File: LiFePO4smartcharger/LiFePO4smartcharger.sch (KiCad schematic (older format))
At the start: 105 parts, among them J1 Conn_01x02, J10 Conn_01x01, J11 Conn_01x01, J12 Conn_01x04, J13 Conn_01x01, J2 Conn_02x03_Odd_Even, J3 Conn_01x02, J4 Conn_01x02, J5 Barrel_Jack, J6 Conn_01x01, J7 Conn_01x01, J8 Conn_01x02, J9 Conn_01x02, Q1 TIP42, Q2 TIP41, Q3 2N3906, Q4 TIP41C, T1 Transformer_1P1Sdotted, U1 ATMEGA328P-PU, U2 LM358, U3 LCD-016N002L, U4 TL494, U9 LM7805_TO220, X3 16MHz

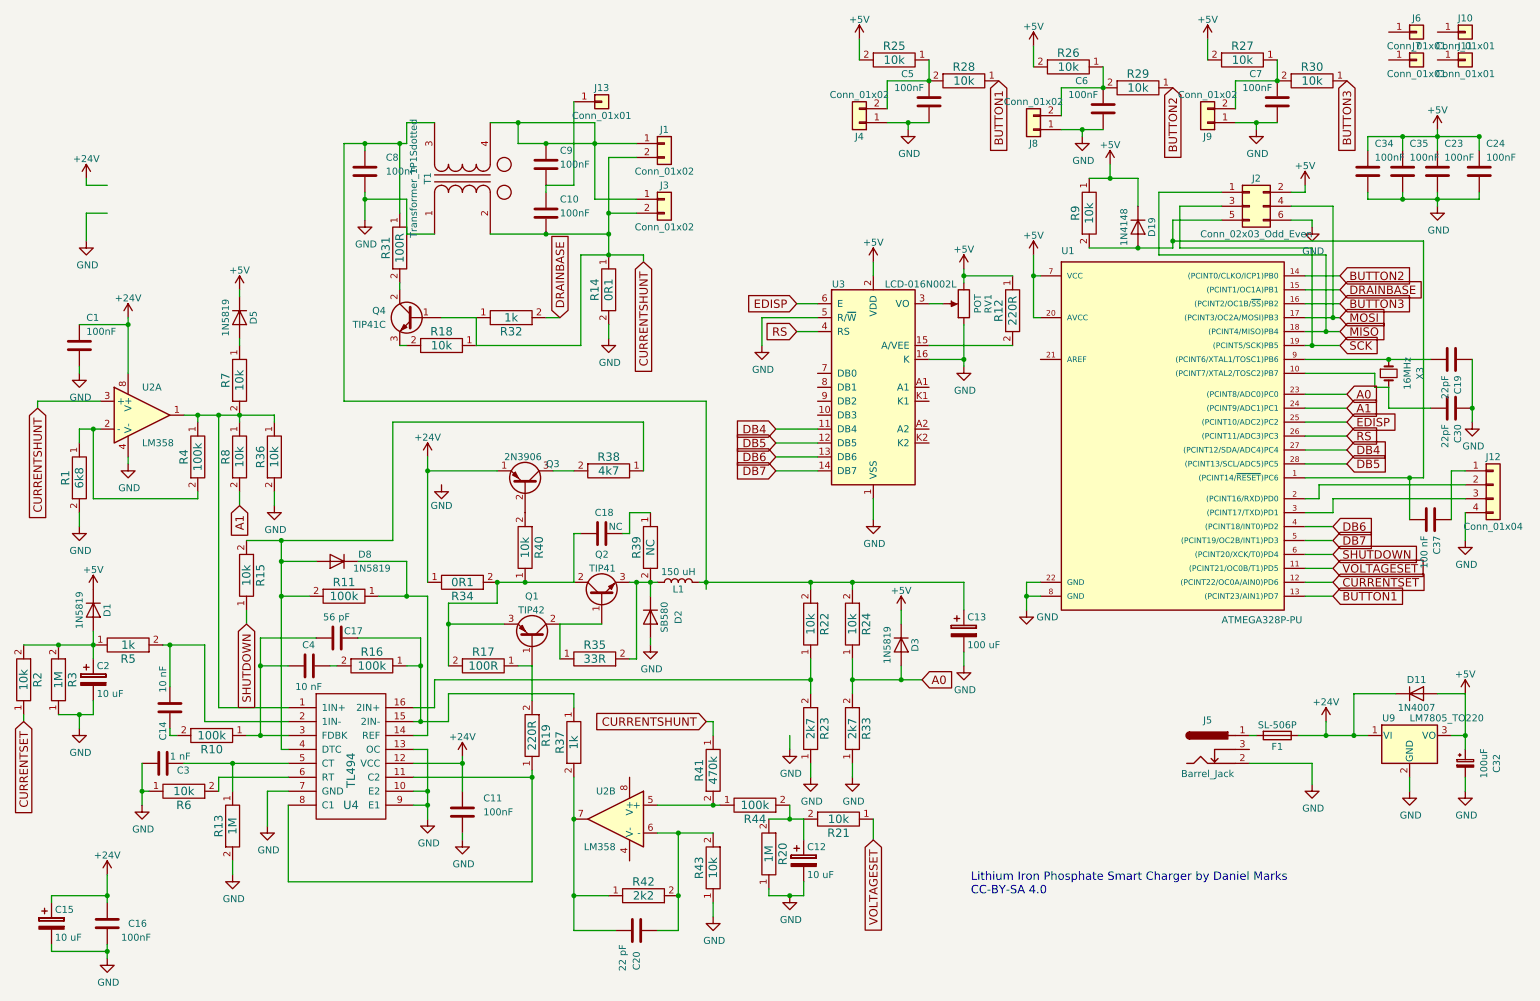
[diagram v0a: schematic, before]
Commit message: JLCPCB 2021-03-26
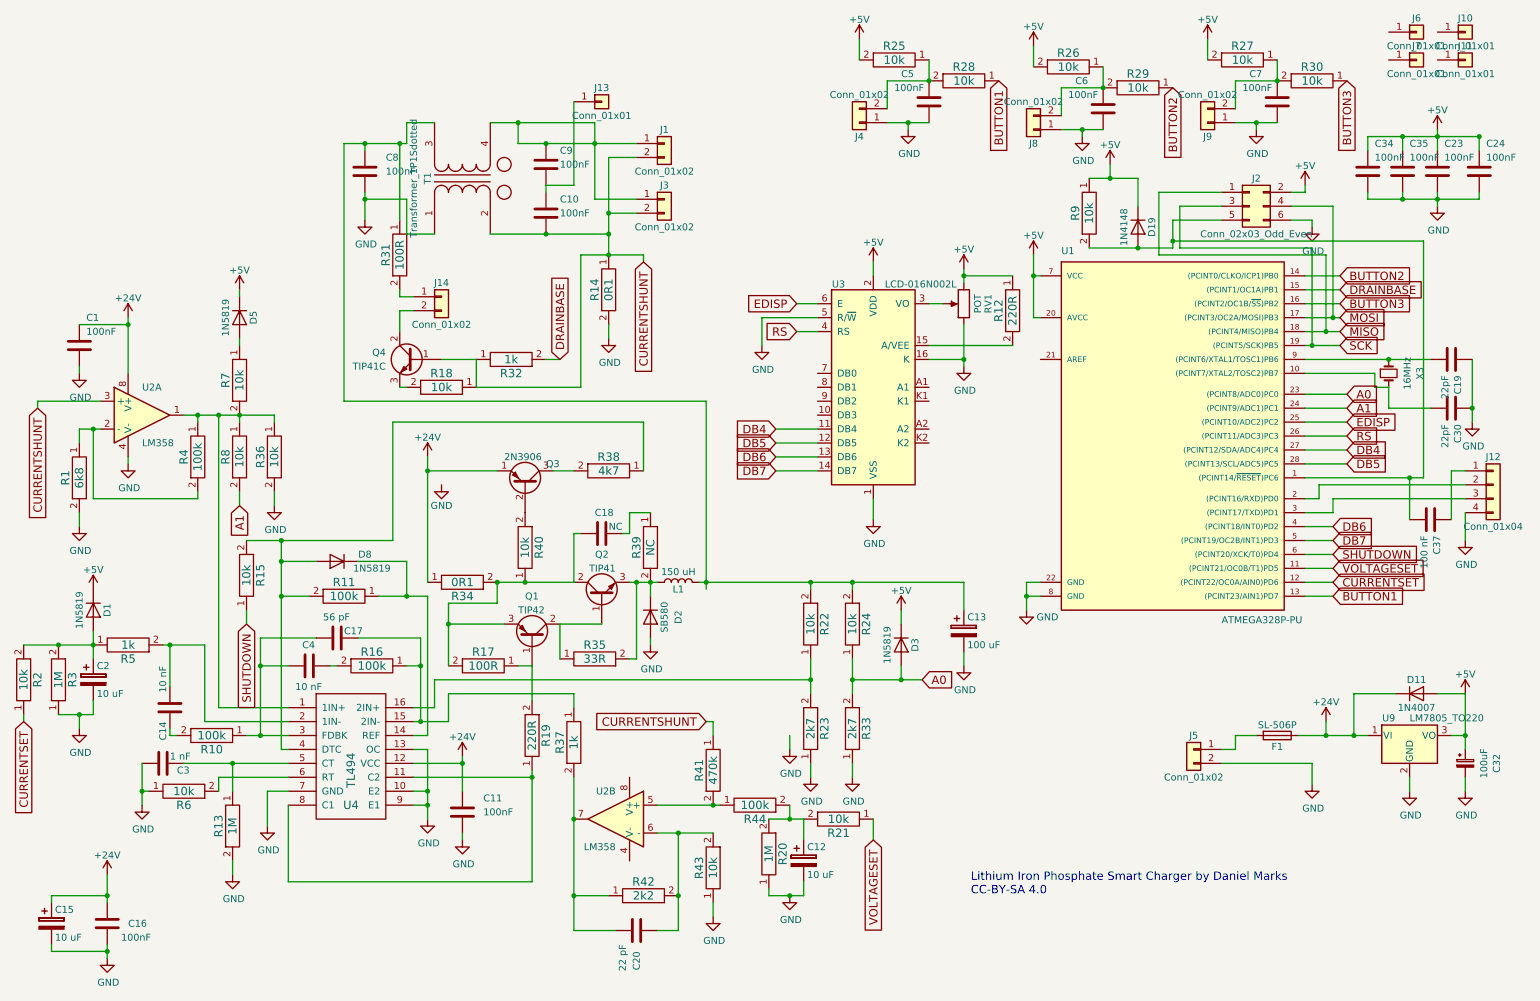
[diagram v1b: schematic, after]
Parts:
- removed J5: Barrel_Jack, Connectors:BARREL_JACK, symbol Barrel_Jack
- added J14, J5: Conn_01x02, Connectors_Terminal_Blocks:TerminalBlock_bornier-2_P5.08mm, symbol Conn_01x02
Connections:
- net GND: now also J5.2 (Pin_2)
- net at F1.2: now also J5.1 (Pin_1)
- net at R31.2: now also J14.1 (Pin_1); no longer Q4.2 (C)
- new net: J14.2 (Pin_2), Q4.2 (C)
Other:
- moved on the sheet: Q4, R18, R31, R32
